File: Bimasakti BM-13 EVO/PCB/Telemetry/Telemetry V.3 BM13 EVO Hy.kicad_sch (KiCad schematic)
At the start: 23 parts, among them J1 MSD-4-A, J2 CON INT/32, J4 Conn_01x16_Pin, U1 ESP32-DEVKIT-V1, U2 74LVC125APW_118, U3 DS3231SN_

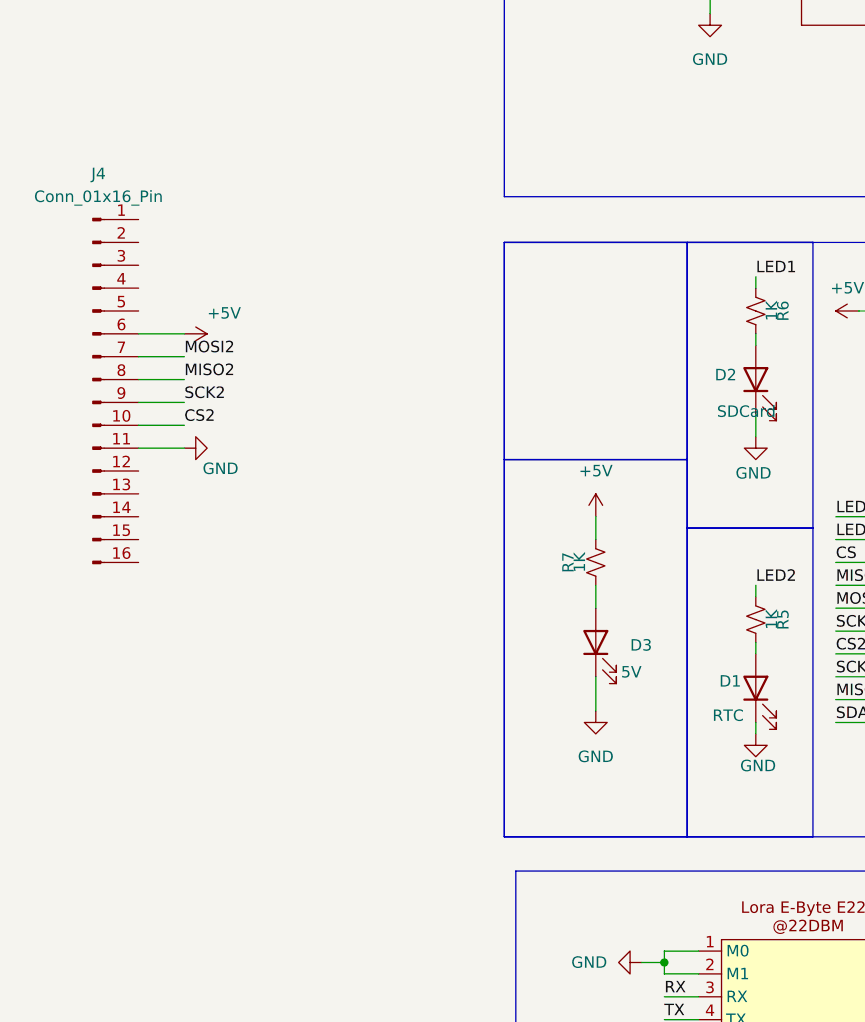
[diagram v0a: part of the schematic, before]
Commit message: Aku Telemetry
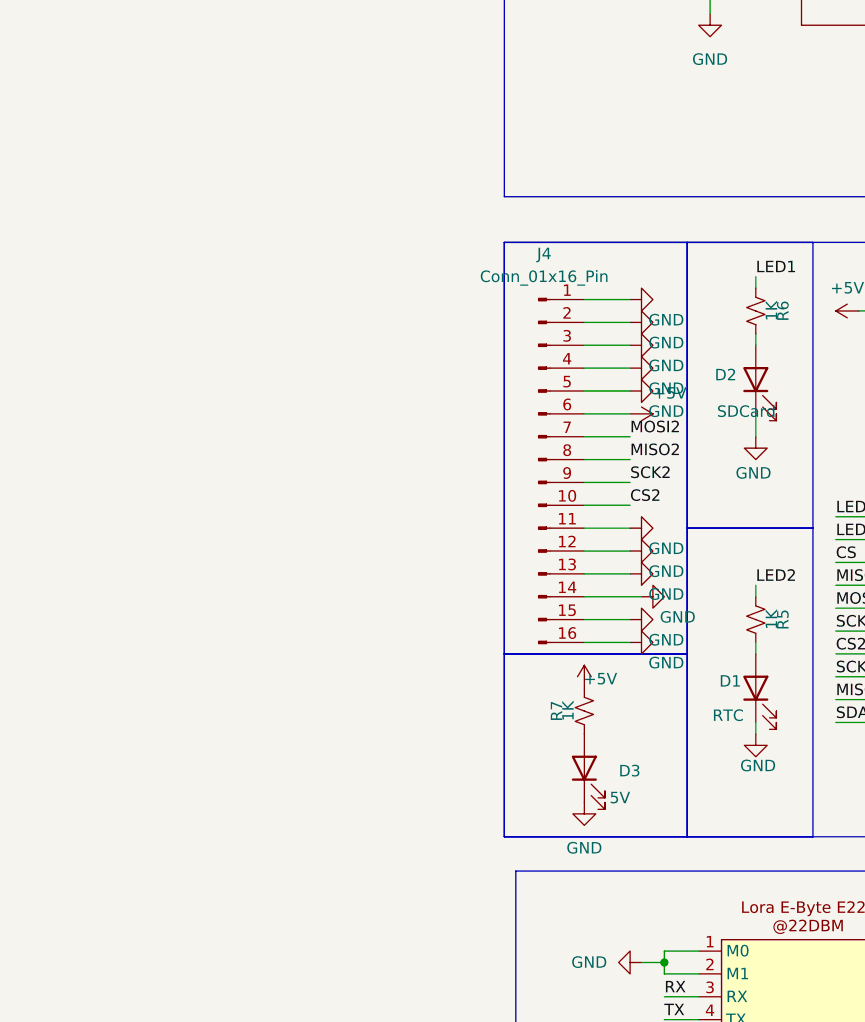
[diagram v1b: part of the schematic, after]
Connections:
- net GND: now also J4.1 (Pin_1), J4.12 (Pin_12), J4.13 (Pin_13), J4.14 (Pin_14), J4.15 (Pin_15), J4.16 (Pin_16), J4.2 (Pin_2), J4.3 (Pin_3), J4.4 (Pin_4), J4.5 (Pin_5)
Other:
- moved on the sheet: D3, J4, R7
